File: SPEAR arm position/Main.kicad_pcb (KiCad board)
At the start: 2 copper layers, 40.6 x 44.5 mm, 6 parts, among them J1 Conn_01x03, U1 Potentiometer

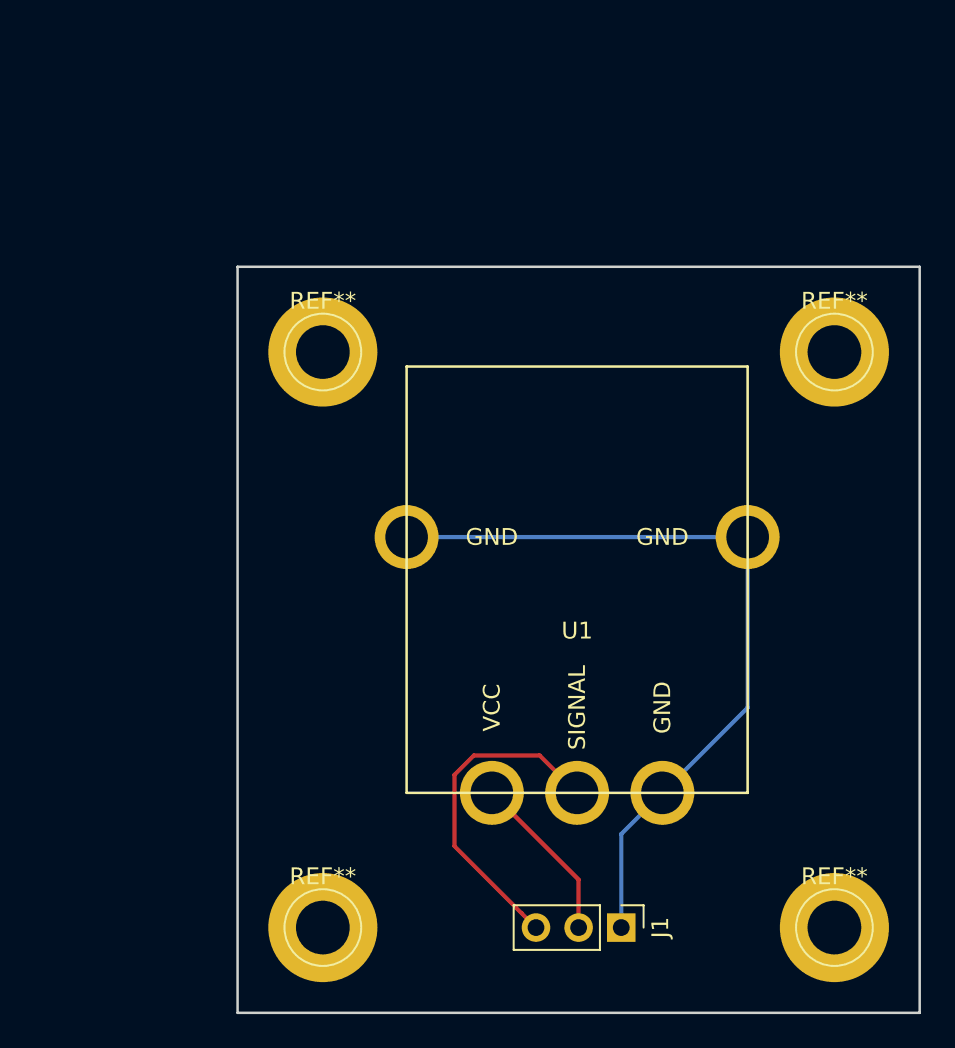
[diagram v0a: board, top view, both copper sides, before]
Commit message: Made some changes to arm position sensor. - Corrected potentiometer footprint. - Made mounting holes and overall size nice numbers (20x35 and 30x45). - Added some silkscreen features.
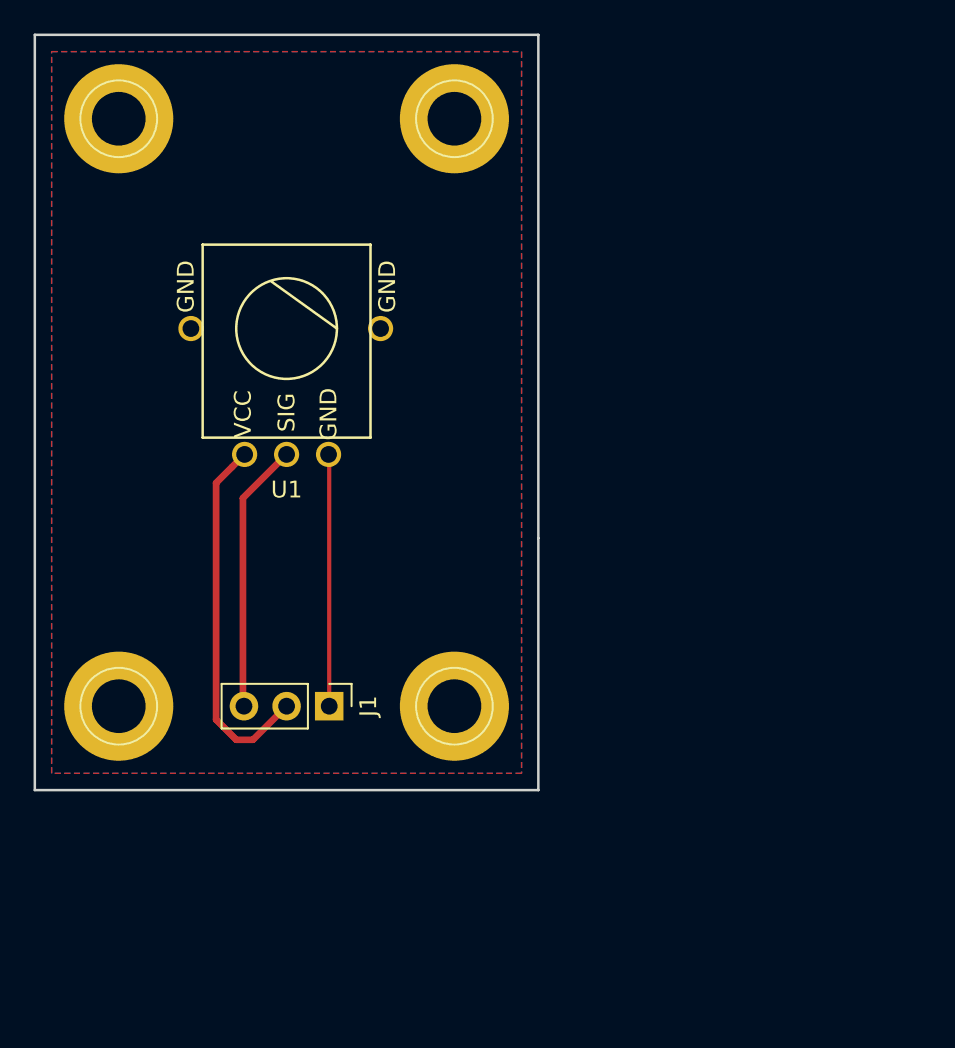
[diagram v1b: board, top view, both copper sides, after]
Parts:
- moved REF** 26.6 mm to (145.0, 75.0)
- moved REF** 26.2 mm to (145.0, 110.0)
- moved U1 22.9 mm to (135.0, 90.0)
- moved J1 21.8 mm to (137.5, 110.0)
- moved REF** 18.5 mm to (125.0, 75.0)
- moved REF** 17.9 mm to (125.0, 110.0)
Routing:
- net /GND: track 46.7 -> 15.0 mm
- net /VCC: track 10.2 -> 22.0 mm
- net /SIGNAL: track 19.8 -> 16.1 mm
- added copper zone on B.Cu, net /GND
- added copper zone on F.Cu, net /GND
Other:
- board size 40.6 x 44.5 mm -> 30 x 45 mm
- board text added: "SIG VCC GND"
- board text added: "SPEAR"
- board text added: "Top"
